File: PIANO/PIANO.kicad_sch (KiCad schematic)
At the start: 31 parts, among them SW1 ON/OFF, SW2 RESET, U1 LF33_TO220, U2 ESP32-WROOM-32U, U3 Opamp_Dual, U4 Opamp_Dual

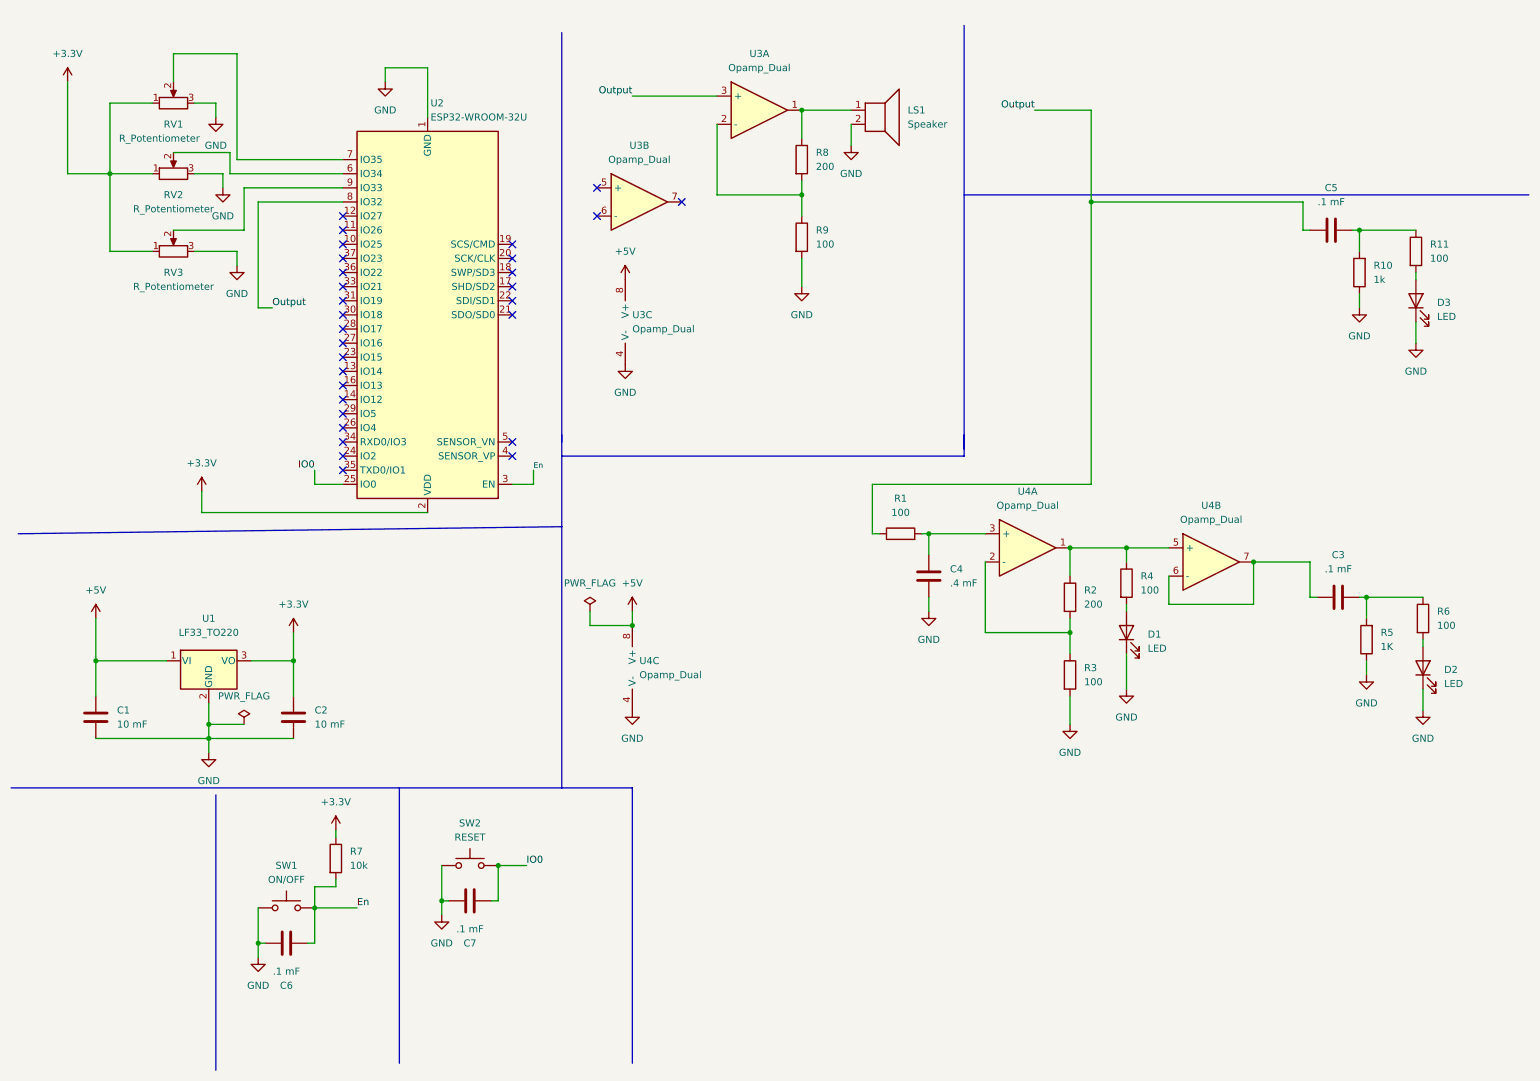
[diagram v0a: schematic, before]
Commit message: dflskdjf
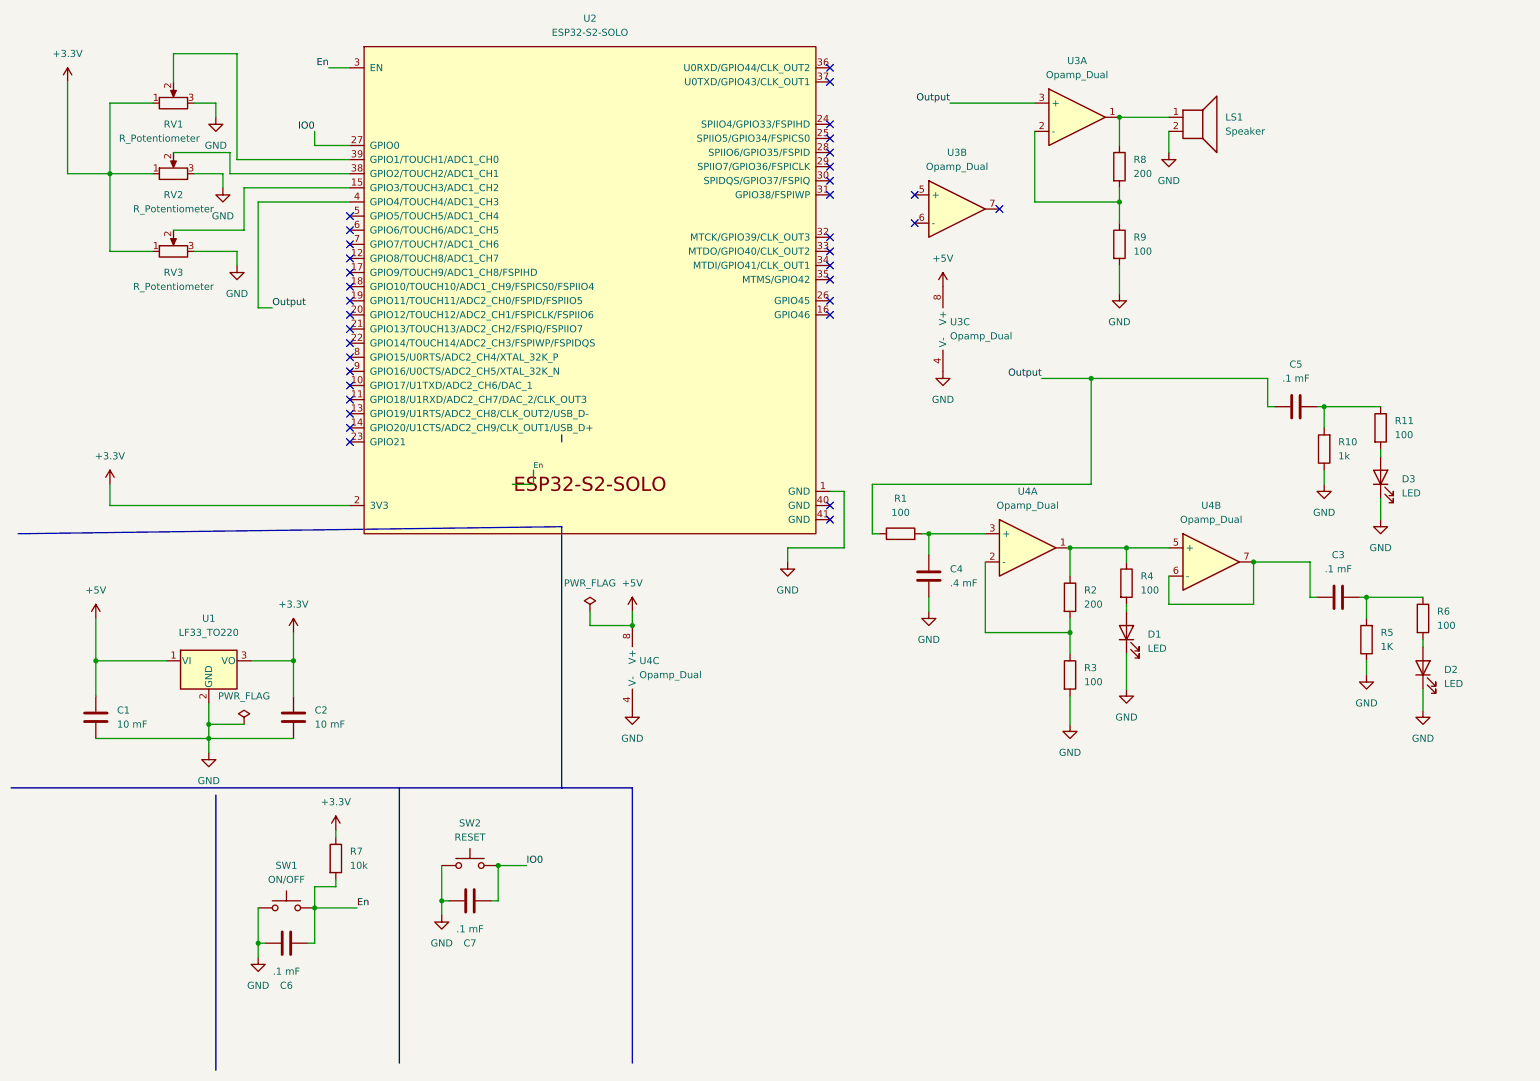
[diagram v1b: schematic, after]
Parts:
- removed U2: ESP32-WROOM-32U, RF_Module:ESP32-WROOM-32U, symbol RF_Module:ESP32-WROOM-32U
- added U2: ESP32-S2-SOLO, Espressif:ESP32-S2-SOLO, symbol Espressif:ESP32-S2-SOLO
- C1, C2: footprint (none) -> Capacitor_SMD:C_0805_2012Metric
- C3, C4, C5, C6, C7: footprint (none) -> Capacitor_SMD:C_0603_1608Metric
- D1, D2, D3: footprint (none) -> LED_THT:LED_D5.0mm-3
- LS1: footprint (none) -> Sensor_Audio:CUI_CMC-4013-SMT
- R1, R11, R2, R3, R4, R6, R8, R9: footprint (none) -> Resistor_SMD:R_0603_1608Metric
- R10, R5, R7: footprint (none) -> Resistor_SMD:R_0805_2012Metric
- RV1, RV2, RV3: footprint (none) -> Potentiometer_THT:Potentiometer_ACP_CA9-V10_Vertical
- SW1, SW2: footprint (none) -> Button_Switch_SMD:SW_DPDT_CK_JS202011JCQN
- U3, U4: footprint (none) -> Library:SOIC127P600X175-8N
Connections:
- net +3V3: now also U2.2 (3V3)
- net En: now also U2.3 (EN)
- net GND: now also U2.1 (GND)
- net IO0: now also U2.27 (GPIO0)
- net Output: now also U2.4 (GPIO4/TOUCH4/ADC1_CH3)
- net at RV2.2: now also U2.38 (GPIO2/TOUCH2/ADC1_CH1)
- net at RV1.2: now also U2.39 (GPIO1/TOUCH1/ADC1_CH0)
- net at RV3.2: now also U2.15 (GPIO3/TOUCH3/ADC1_CH2)
- no-connect marks 30 -> 36
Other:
- moved on the sheet: C5, D3, LS1, R10, R11, R8, R9, U3A, U3B, U3C
